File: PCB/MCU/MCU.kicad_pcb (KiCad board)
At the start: 2 copper layers, 40 x 46.2 mm, 35 parts, among them IC1 TMP112NAIDRLR, J1 Conn_02x06_Odd_Even, J2 Conn_02x06_Odd_Even, J3 USB_B_Micro, J4 Programmer, SW1 SW_Push, U1 MPU6050, U2 MDBT50Q-1MV2, U3 MAX6372, Y1 32.768kHz

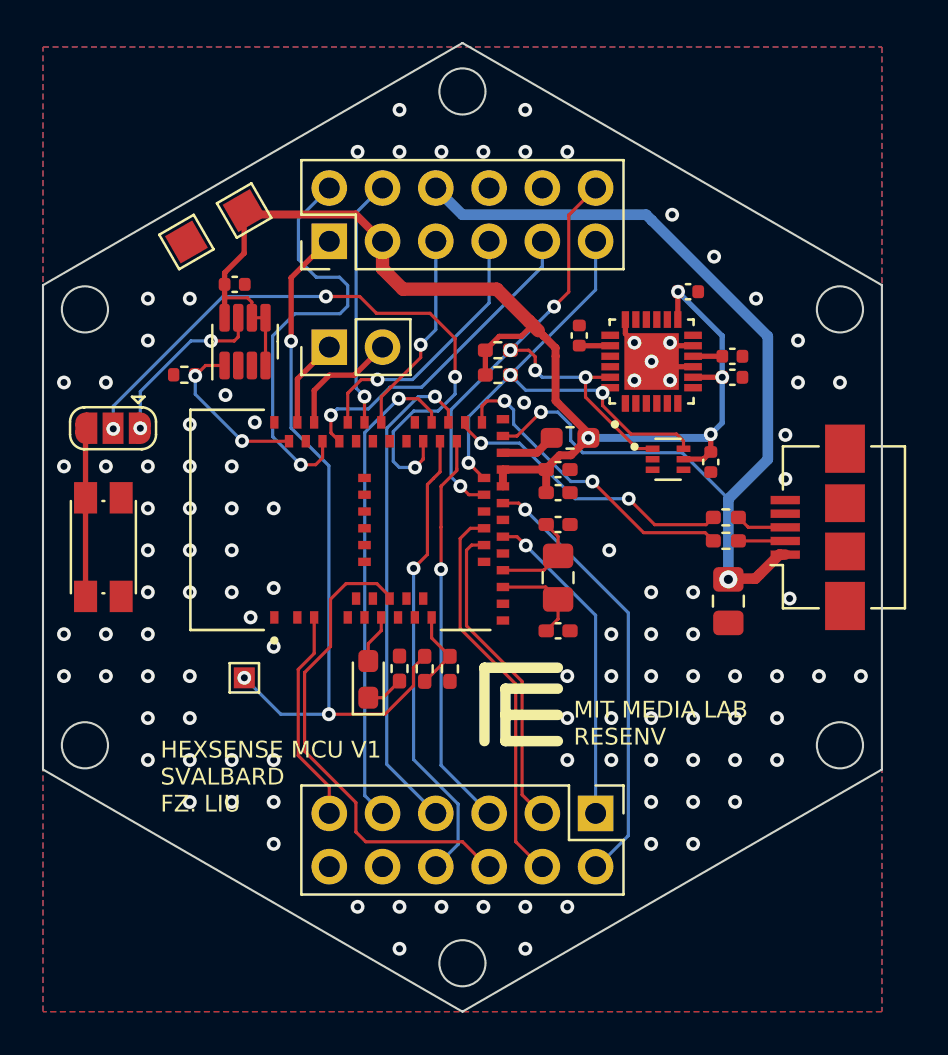
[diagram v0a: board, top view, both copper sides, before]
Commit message: udated by FZ
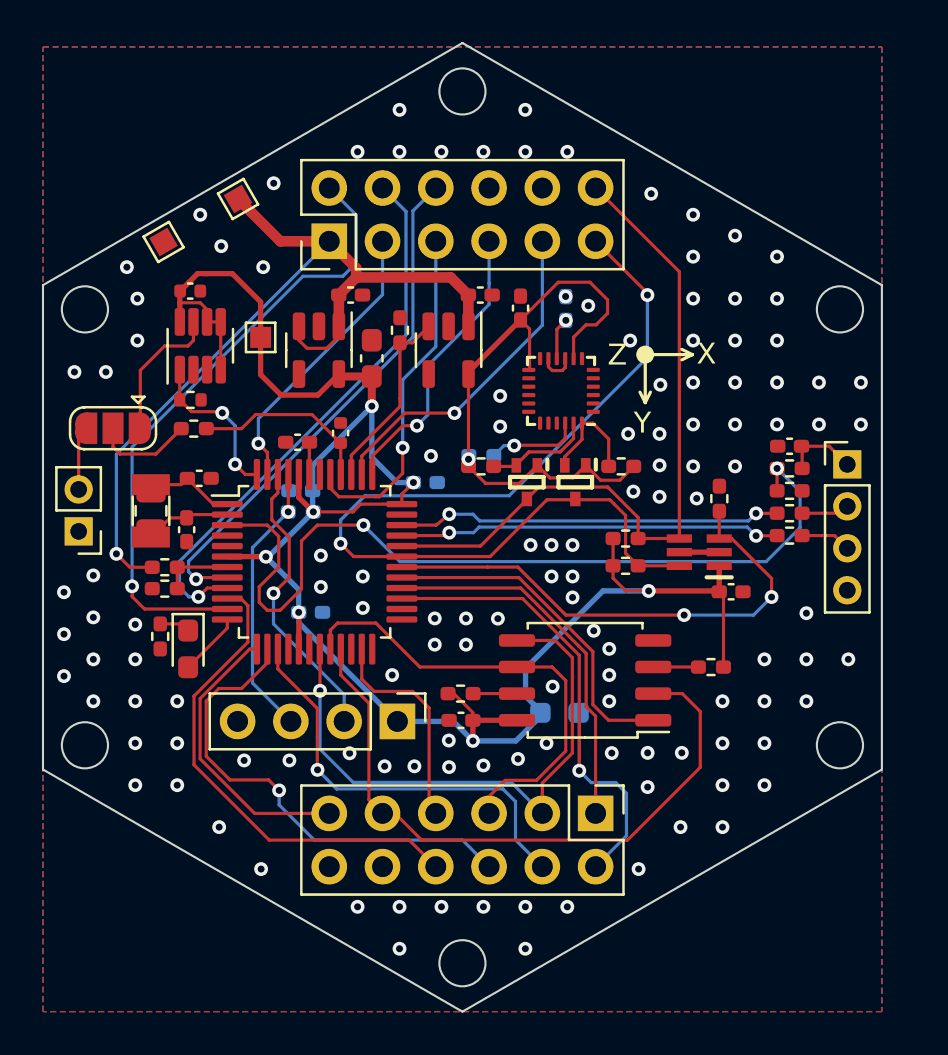
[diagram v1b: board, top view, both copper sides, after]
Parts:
- removed IC1: TMP112NAIDRLR, Mylib:SOT50P160X60-6N
- removed J3: USB_B_Micro, Connector_USB:USB_Micro-B_Amphenol_10104110_Horizontal
- removed L1: 10uH, Inductor_SMD:L_0603_1608Metric_Pad1.05x0.95mm_HandSolder
- removed SW1: SW_Push, Button_Switch_SMD:SW_Push_1P1T_NO_CK_KMR2
- added C12: 1uF, Capacitor_SMD:C_0402_1005Metric_Pad0.74x0.62mm_HandSolder, F.Cu at (142.3, 96.0)
- added C13: 10pF, Capacitor_SMD:C_0402_1005Metric, F.Cu at (144.3, 95.6)
- added C14: 0.1uF, Capacitor_SMD:C_0402_1005Metric_Pad0.74x0.62mm_HandSolder, F.Cu at (151.0, 89.0)
- added C15: 0.1uF, Capacitor_SMD:C_0402_1005Metric_Pad0.74x0.62mm_HandSolder, B.Cu at (142.4, 98.4)
- added C16: 0.1uF, Capacitor_SMD:C_0402_1005Metric_Pad0.74x0.62mm_HandSolder, B.Cu at (155.1, 89.7)
- added IC2: LTC4311CSC6#TRPBF, SamacSys_Parts:SOT65P210X100-6N, F.Cu at (161.5, 101.3)
- added J5: RESET, Connector_PinHeader_2.00mm:PinHeader_1x02_P2.00mm_Vertical, F.Cu at (131.9, 100.3)
- added J6: Conn_01x04_Pin, Connector_PinHeader_2.00mm:PinHeader_1x04_P2.00mm_Vertical, F.Cu at (168.5, 97.1)
- added Q1: RUM002N02T2L, SamacSys_Parts:SOTFL50P160X60-3N, F.Cu at (155.5, 98.0)
- added Q2: RUM002N02T2L, SamacSys_Parts:SOTFL50P160X60-3N, F.Cu at (153.2, 98.0)
- added R10: 10k, Resistor_SMD:R_0402_1005Metric_Pad0.72x0.64mm_HandSolder, B.Cu at (142.4, 99.4)
- added R12: 10K, Resistor_SMD:R_0402_1005Metric_Pad0.72x0.64mm_HandSolder, F.Cu at (150.1, 108.0)
- added R13: 10K, Resistor_SMD:R_0402_1005Metric_Pad0.72x0.64mm_HandSolder, F.Cu at (162.0, 106.8)
- added R14: 499K, Resistor_SMD:R_0402_1005Metric_Pad0.72x0.64mm_HandSolder, F.Cu at (165.8, 97.3)
- added R15: 499K, Resistor_SMD:R_0402_1005Metric_Pad0.72x0.64mm_HandSolder, F.Cu at (165.8, 98.4)
- added R16: 10K, Resistor_SMD:R_0402_1005Metric_Pad0.72x0.64mm_HandSolder, F.Cu at (147.2, 90.7)
- added R17: 10K, Resistor_SMD:R_0402_1005Metric_Pad0.72x0.64mm_HandSolder, F.Cu at (151.0, 97.2)
- added R18: 10K, Resistor_SMD:R_0402_1005Metric_Pad0.72x0.64mm_HandSolder, F.Cu at (157.7, 97.2)
- added R19: PH, Resistor_SMD:R_0805_2012Metric_Pad1.20x1.40mm_HandSolder, F.Cu at (135.3, 99.3)
- added R20: 10K, Resistor_SMD:R_0603_1608Metric_Pad0.98x0.95mm_HandSolder, B.Cu at (154.8, 108.9)
- added R21: 10K, Resistor_SMD:R_0402_1005Metric_Pad0.72x0.64mm_HandSolder, B.Cu at (151.1, 96.7)
- added R3: 10K, Resistor_SMD:R_0402_1005Metric_Pad0.72x0.64mm_HandSolder, F.Cu at (162.4, 98.7)
- added R9: 330, Resistor_SMD:R_0402_1005Metric_Pad0.72x0.64mm_HandSolder, F.Cu at (137.3, 95.4)
- added U4: ADP160AUJZ-3.3-R7, Package_TO_SOT_SMD:TSOT-23-5, F.Cu at (143.3, 91.7)
- added U5: ICM-20948, Sensor_Motion:InvenSense_QFN-24_3x3mm_P0.4mm, F.Cu at (154.9, 93.6)
- added U6: ADP160AUJZ-1.8, Package_TO_SOT_SMD:TSOT-23-5, F.Cu at (149.5, 91.7)
- C1, C7: value 0.1uF -> 0.01uF; footprint Capacitor_SMD:C_0402_1005Metric -> Capacitor_SMD:C_0402_1005Metric_Pad0.74x0.62mm_HandSolder
- C11: footprint Capacitor_SMD:C_0402_1005Metric -> Capacitor_SMD:C_0402_1005Metric_Pad0.74x0.62mm_HandSolder
- C2, C4: value 22pF -> 18pF
- C3: value 10000pF -> 0.01uF; footprint Capacitor_SMD:C_0402_1005Metric -> Capacitor_SMD:C_0402_1005Metric_Pad0.74x0.62mm_HandSolder
- C5: value 10uF -> 1uF; moved to B.Cu
- C6: value 10uF -> 0.1uF; moved to B.Cu
- C8: value 2200pF -> 0.1uF; footprint Capacitor_SMD:C_0402_1005Metric -> Capacitor_SMD:C_0402_1005Metric_Pad0.74x0.62mm_HandSolder
- C9: value 47uF -> 10uF; footprint Capacitor_SMD:C_0805_2012Metric_Pad1.18x1.45mm_HandSolder -> Capacitor_SMD:C_0603_1608Metric_Pad1.08x0.95mm_HandSolder
- J4: value Programmer -> Conn_01x04_Pin; footprint Connector_PinHeader_2.54mm:PinHeader_1x02_P2.54mm_Vertical -> Connector_PinHeader_2.54mm:PinHeader_1x04_P2.54mm_Vertical
- TP1: value VCC_TP -> BAT_TP; footprint TestPoint:TestPoint_Pad_1.5x1.5mm -> TestPoint:TestPoint_Pad_1.0x1.0mm
- TP2: value GND_TP -> BAT_TP; footprint TestPoint:TestPoint_Pad_1.5x1.5mm -> TestPoint:TestPoint_Pad_1.0x1.0mm
- U1: value MPU6050 -> MB85RS2MTAPNF-G-BDERE1; footprint Mylib:IC_MPU6050 -> Package_SO:SSOP-8_5.25x5.24mm_P1.27mm
- U2: value MDBT50Q-1MV2 -> ATSAMD21G18A-A; footprint Mylib:XCVR_MDBT50Q-1MV2 -> Package_QFP:TQFP-48_7x7mm_P0.5mm
- Y1: value 32.768kHz -> 32KHz; footprint Capacitor_SMD:C_0805_2012Metric_Pad1.18x1.45mm_HandSolder -> Crystal:Crystal_SMD_3215-2Pin_3.2x1.5mm
- moved TP3 22.8 mm to (139.5, 84.4), turned to 30 degrees
- moved C3 20.9 mm to (150.1, 109.3)
- moved C9 20.6 mm to (145.8, 92.0)
- moved Y1 19.7 mm to (135.3, 99.3)
- moved C2 18.6 mm to (137.6, 97.8)
- moved J4 18.1 mm to (147.1, 109.4), turned to -90 degrees
- moved C4 17.7 mm to (137.0, 100.2), turned to 90 degrees
- moved U1 15.5 mm to (156.0, 107.4), turned to 180 degrees
- moved C1 14.5 mm to (163.0, 103.2), turned to 0 degrees
- moved R8 14.1 mm to (136.0, 103.0), turned to 180 degrees
- moved R7 13.3 mm to (136.0, 102.0), turned to 0 degrees
- moved C6 13.1 mm to (142.9, 104.2)
- moved R2 11.9 mm to (157.9, 101.9)
- moved C11 11.7 mm to (152.9, 89.6), turned to 90 degrees
- moved R11 11.5 mm to (135.8, 105.3), turned to -90 degrees
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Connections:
- C1 pad 1: GND -> VCC
- C1 pad 2: VCC -> GND
- C11 pad 1: VCC -> +1V8
- C2 pad 2: Net-(U2-P0.00/XL1) -> Net-(U2-PA00)
- C3 pad 1: GND -> VCC
- C3 pad 2: VCC -> GND
- C4 pad 2: Net-(U2-P0.01/XL2) -> Net-(U2-PA01)
- C7 pad 1: GND -> +5V
- C7 pad 2: Net-(U1-REGOUT) -> GND
- C8 pad 1: GND -> /VBAT
- C8 pad 2: Net-(U1-CPOUT) -> GND
- C9 pad 1: +5V -> GND
- C9 pad 2: GND -> VCC
- D1 pad 2: /LED1 -> /D9
- J1 pad 2: /~{EN} -> /D8
- J1 pad 3: VCC -> /A5
- J1 pad 4: /VBAT_OK -> /A3
- J1 pad 5: /~{I2C_RESET} -> /MPPT_EN
- J1 pad 6: +5V -> /A2
- J2 pad 1: /D11 -> /D12
- J2 pad 11: /LED2 -> /D4
- J2 pad 2: /D13 -> /D10
- J2 pad 3: /A1 -> /MOSI
- J2 pad 4: /D6 -> /D1
- J2 pad 6: /A5 -> /D3
- J2 pad 7: /MOSI -> /D2
- J2 pad 8: /~{CS} -> /A4
- J4 pad 1: /SWDCLK -> VCC
- JP1 pad 2: /~{RESET} -> Net-(JP1-C)
- R1 pad 1: /SDA -> /SCL
- R2 pad 1: /SCL -> /SDA
- R4 pad 1: /D2 -> /RXLED
- R7 pad 2: /A2 -> /A1
- R8 pad 1: /A2 -> /A1
- U1 pad 1: unconnected-(U1-CLKIN-Pad1) -> /D6
- U1 pad 2: unconnected-(U1-NC2-Pad2) -> /MISO
- U1 pad 3: unconnected-(U1-NC3-Pad3) -> Net-(U1-~{WP})
- U1 pad 4: unconnected-(U1-NC4-Pad4) -> GND
- U1 pad 5: unconnected-(U1-NC5-Pad5) -> /MOSI
- U1 pad 6: unconnected-(U1-AUX_DA-Pad6) -> /SCK
- U1 pad 7: unconnected-(U1-AUX_CL-Pad7) -> Net-(U1-~{HOLD})
- U2 pad 1: GND -> Net-(U2-PA00)
- U2 pad 10: unconnected-(U2-P0.29/AIN5-Pad10) -> /A4
- U2 pad 11: /A4 -> /D8
- U2 pad 12: unconnected-(U2-P0.31/AIN7-Pad12) -> /D9
- U2 pad 13: /A3 -> /D4
- U2 pad 14: /A2 -> /D3
- U2 pad 15: GND -> /D1
- U2 pad 16: /D10 -> /D0
- U2 pad 17: Net-(U2-P0.00/XL1) -> VCC
- U2 pad 18: Net-(U2-P0.01/XL2) -> GND
- U2 pad 19: /D9 -> /MOSI
- U2 pad 2: GND -> Net-(U2-PA01)
- U2 pad 20: /A0 -> /SCK
- U2 pad 21: /A1 -> /MISO
- U2 pad 22: /D11 -> unconnected-(U2-PA13-Pad22)
- U2 pad 23: /D6 -> /D2
- U2 pad 24: /D12 -> /D5
- U2 pad 25: /D5 -> /D11
- U2 pad 27: /SCL -> /D10
- U2 pad 28: VCC -> /D12
- U2 pad 29: /SDA -> /D6
- U2 pad 3: /LED2 -> /A0
- U2 pad 30: VCC -> /D7
- U2 pad 31: Net-(U2-DCCH) -> /SDA
- U2 pad 32: +5V -> /SCL
- U2 pad 33: GND -> /USB-
- U2 pad 34: /USB- -> /USB+
- U2 pad 35: /USB+ -> GND
- U2 pad 36: /SCK -> VCC
- U2 pad 37: /MOSI -> /RXD
- U2 pad 38: /~{CS} -> /TXD
- U2 pad 39: /MISO -> /1V8_EN
- U2 pad 41: unconnected-(U2-P0.17-Pad41) -> /MPPT_EN
- U2 pad 42: unconnected-(U2-P0.19-Pad42) -> GND
- U2 pad 43: unconnected-(U2-P0.21-Pad43) -> Net-(U2-VDDCORE)
- U2 pad 44: /~{I2C_RESET} -> VCC
- U2 pad 45: unconnected-(U2-P0.23-Pad45) -> /SWDCLK
- U2 pad 46: /VBAT_OK -> /SWDIO
- U2 pad 47: unconnected-(U2-P1.00/TRACEDATA0-Pad47) -> /A5
- U2 pad 48: /RXD -> /RXLED
- U2 pad 5: unconnected-(U2-P1.12-Pad5) -> GND
- U2 pad 6: unconnected-(U2-P1.13-Pad6) -> VCC
- U2 pad 7: unconnected-(U2-P1.14-Pad7) -> /A1
- U2 pad 8: /LED1 -> /A2
- U2 pad 9: /A5 -> /A3
- U3 pad 1: /D2 -> /RXLED
- Y1 pad 1: Net-(U2-P0.01/XL2) -> Net-(U2-PA01)
- Y1 pad 2: Net-(U2-P0.00/XL1) -> Net-(U2-PA00)
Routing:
- net +5V: track 47.7 -> 3.61 mm, vias 2 -> 0
- net /A0: track 0.00 -> 40.9 mm, vias 0 -> 2
- net /D8: track 0.00 -> 30.3 mm, vias 0 -> 1
- net VCC: track 63.3 -> 92.8 mm, vias 4 -> 7
- net +1V8: track 0.00 -> 29.2 mm, vias 0 -> 1
- net /A3: track 0.00 -> 26.6 mm, vias 0 -> 1
- net /D10: track 0.00 -> 24.6 mm, vias 0 -> 1
- net /D7: track 0.00 -> 24.4 mm, vias 0 -> 2
- net /A4: track 0.00 -> 23.3 mm
- net /D3: track 0.00 -> 23.0 mm, vias 0 -> 1
- net /~{CS}: track 22.1 -> 0.00 mm, vias 1 -> 0
- net /~{RESET}: track 30.7 -> 8.74 mm, vias 4 -> 0
- net /A2: track 3.92 -> 25.2 mm, vias 0 -> 1
- net /D13: track 21.0 -> 0.00 mm, vias 1 -> 0
- net /SDA: track 24.5 -> 45.4 mm, vias 3 -> 2
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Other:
- board text added: "Fangzhegn Liu MIT Media Lab fzliu@mit.edu"
- board text added: "HexSense Canary Islands"
- board text removed: "HEXSENSE MCU V1 SVALBARD FZ. LIU"
- board text removed: "MIT MEDIA LAB RESENV"
